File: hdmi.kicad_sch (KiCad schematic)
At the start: 41 parts, among them J7 685119136923, Q2 PJE138K, Q3 PJE138K, U12 NTS0102, U13 TPD4E05U06QDQARQ1, U14 TPD4E05U06QDQARQ1, U15 TPD4E05U06QDQARQ1

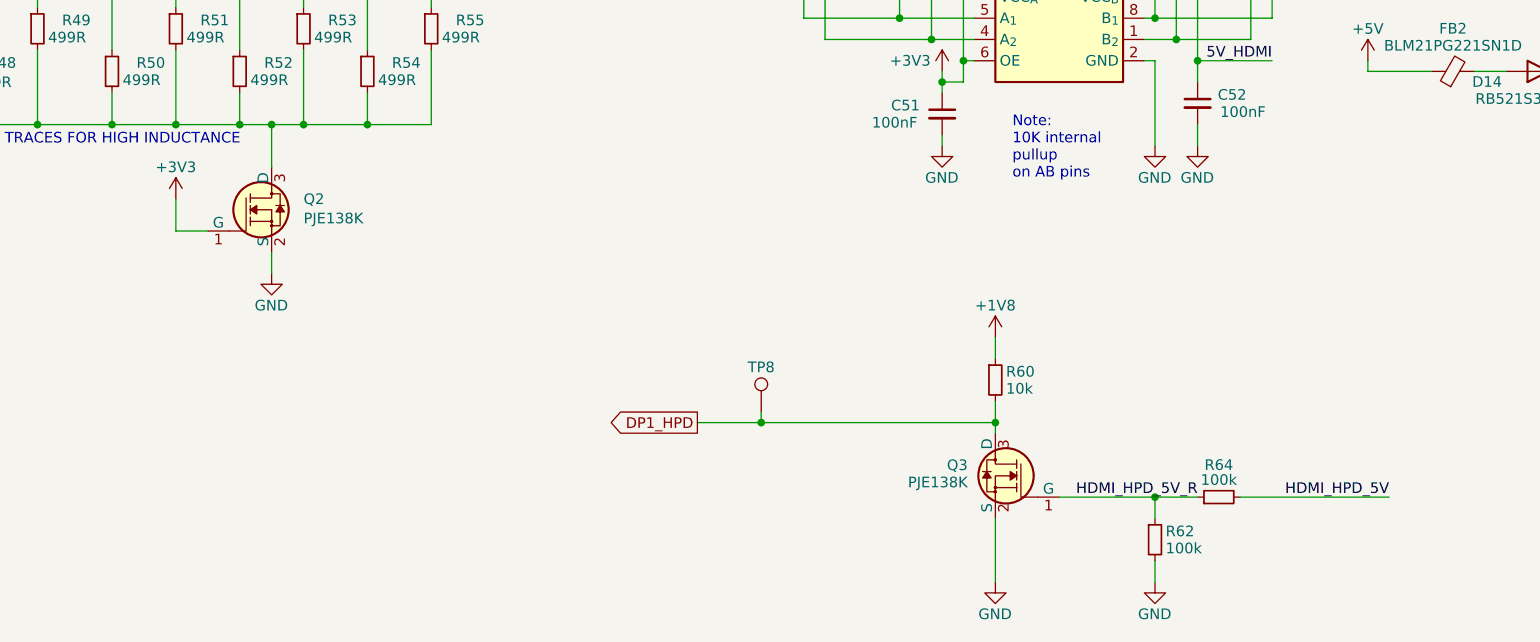
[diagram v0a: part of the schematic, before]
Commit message: Final cleanup, production files
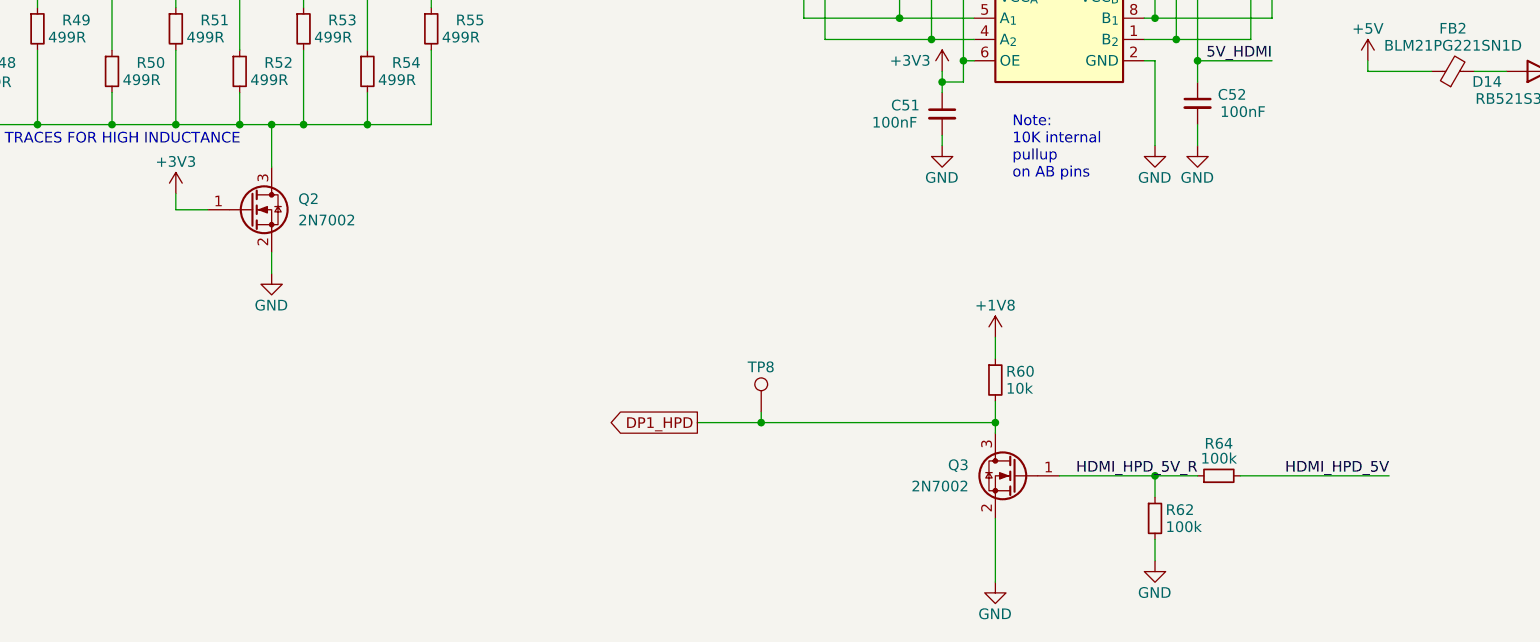
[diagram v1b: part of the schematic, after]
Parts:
- removed Q2, Q3: PJE138K, Package_TO_SOT_SMD:SOT-523, symbol JetsonCarrier:PJE138K
- added Q2, Q3: 2N7002, Package_TO_SOT_SMD:SOT-23, symbol Transistor_FET:2N7002
- FB2: footprint Inductor_SMD:L_0603_1608Metric -> Inductor_SMD:L_0805_2012Metric
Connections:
- net +3V3: now also Q2.1 (G)
- net DP1_HPD: now also Q3.3 (D)
- net GND: now also Q2.2 (S), Q3.2 (S)
- net HDMI_HPD_5V_R: now also Q3.1 (G)
- net at R48.2, R49.2, R50.2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: now also Q2.3 (D)
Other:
- moved on the sheet: R62, R64

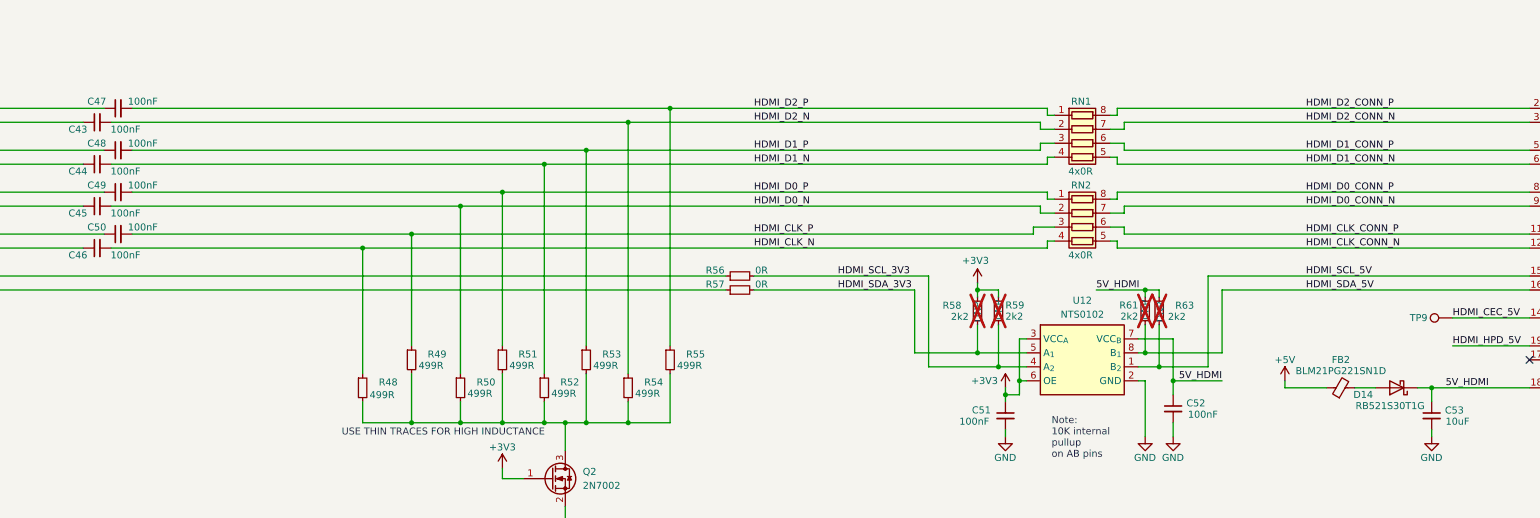
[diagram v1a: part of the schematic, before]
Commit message: Final BOM changes, gerbers
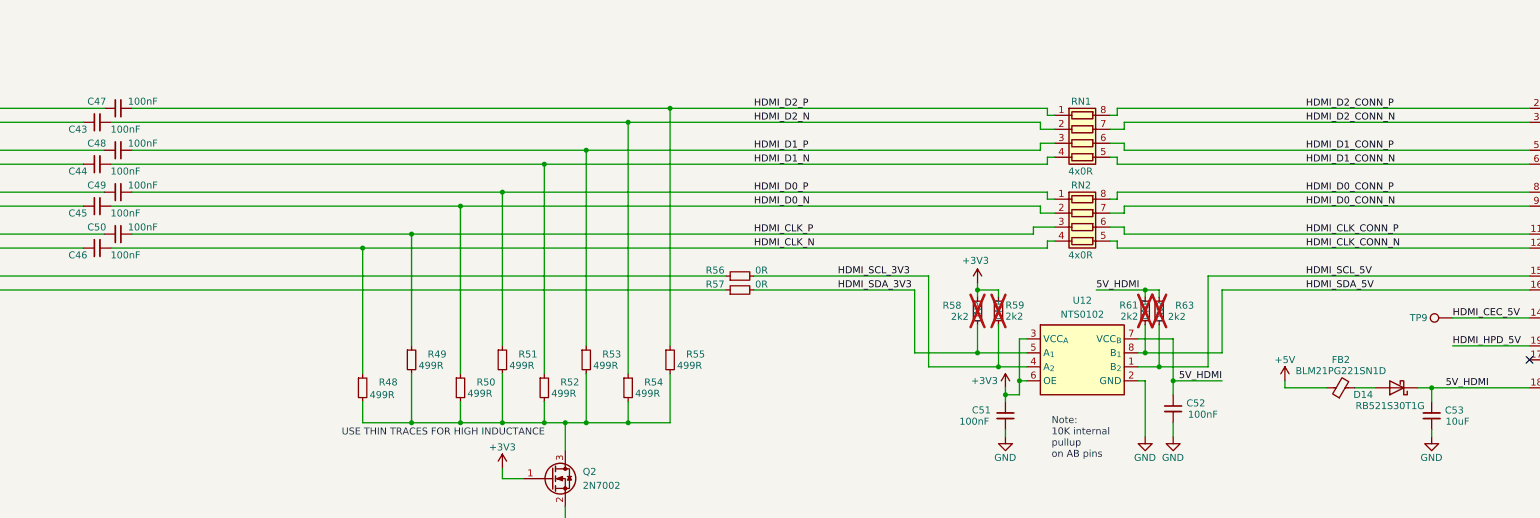
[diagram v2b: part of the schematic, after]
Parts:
- C43, C44, C45, C46, C47, C48, C49, C50: LCSC (none) -> C307331
- C51, C52: LCSC (none) -> C14663
- C53: LCSC (none) -> C96446
- D14: LCSC (none) -> C145179
- FB2: LCSC (none) -> C85840
- J7: LCSC (none) -> C2961651
- Q2, Q3: LCSC (none) -> C8545
- R48, R49, R50, R51, R52, R53, R54, R55: LCSC (none) -> C4125
- R56, R57: LCSC (none) -> C17168
- R58, R59, R61, R63: LCSC (none) -> C25879
- R60: LCSC (none) -> C25804
- R62, R64: LCSC (none) -> C25803
- RN1, RN2: LCSC (none) -> C2001
- U12: LCSC (none) -> C2687851
- U13, U14, U15: LCSC (none) -> C81353
